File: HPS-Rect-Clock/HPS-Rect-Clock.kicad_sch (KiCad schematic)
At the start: 22 parts, among them J1 Conn_01x06, J2 PJ-102AH, Y1 Crystal_16MHz

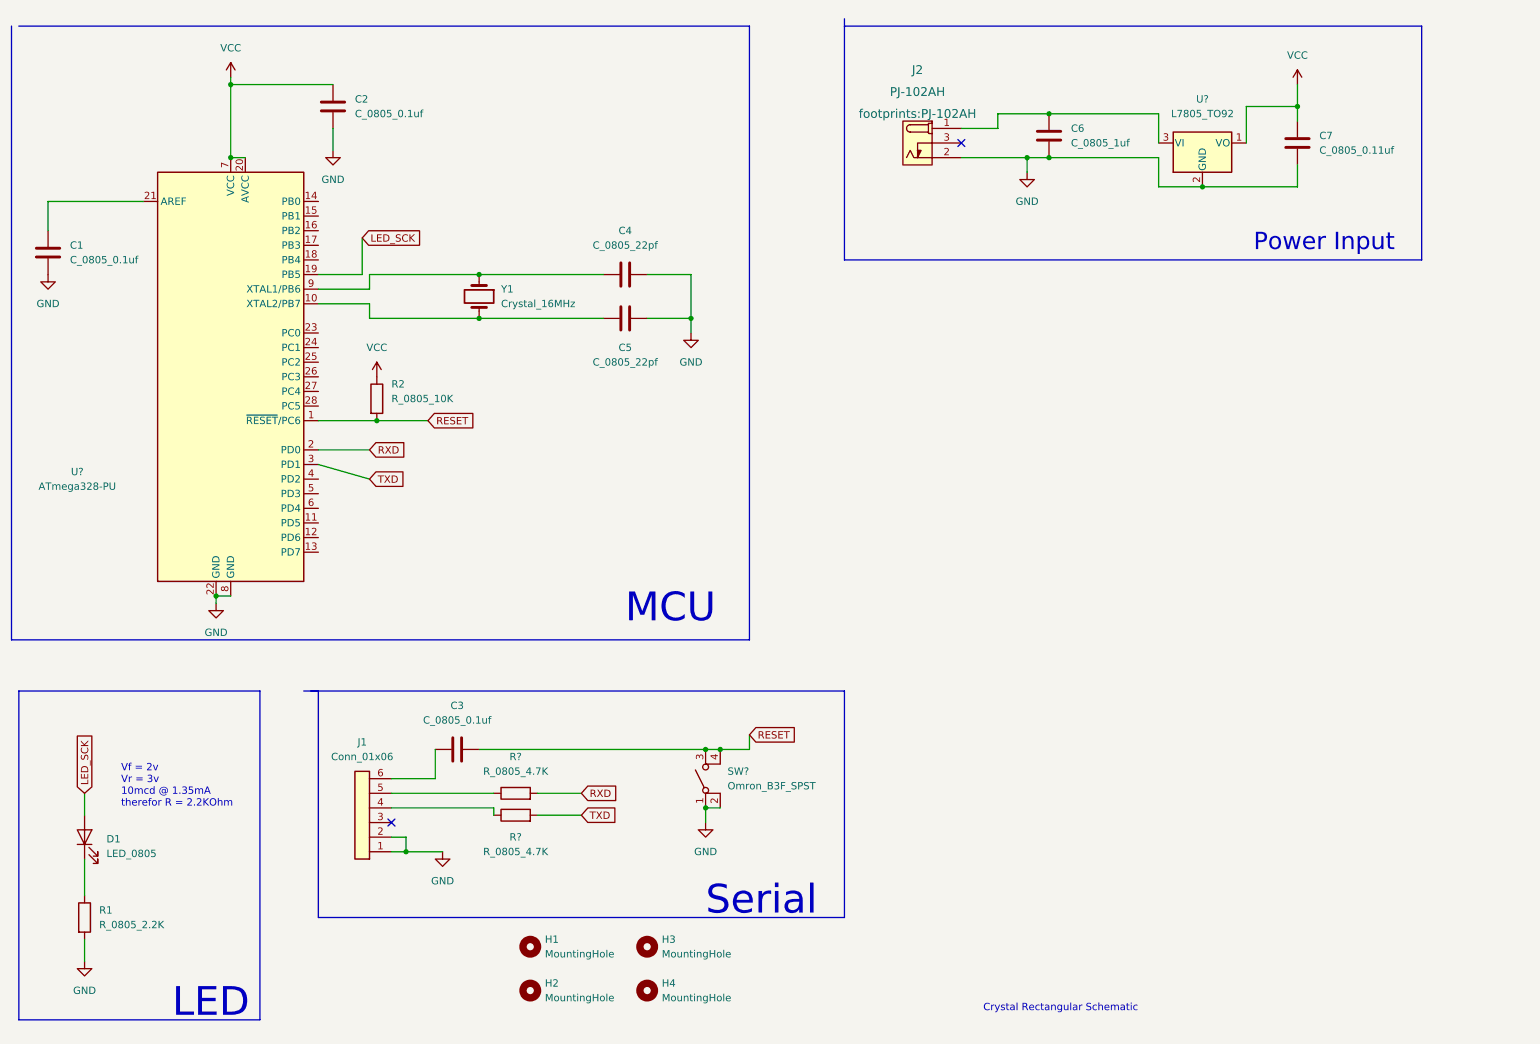
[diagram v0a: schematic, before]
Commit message: Week 3
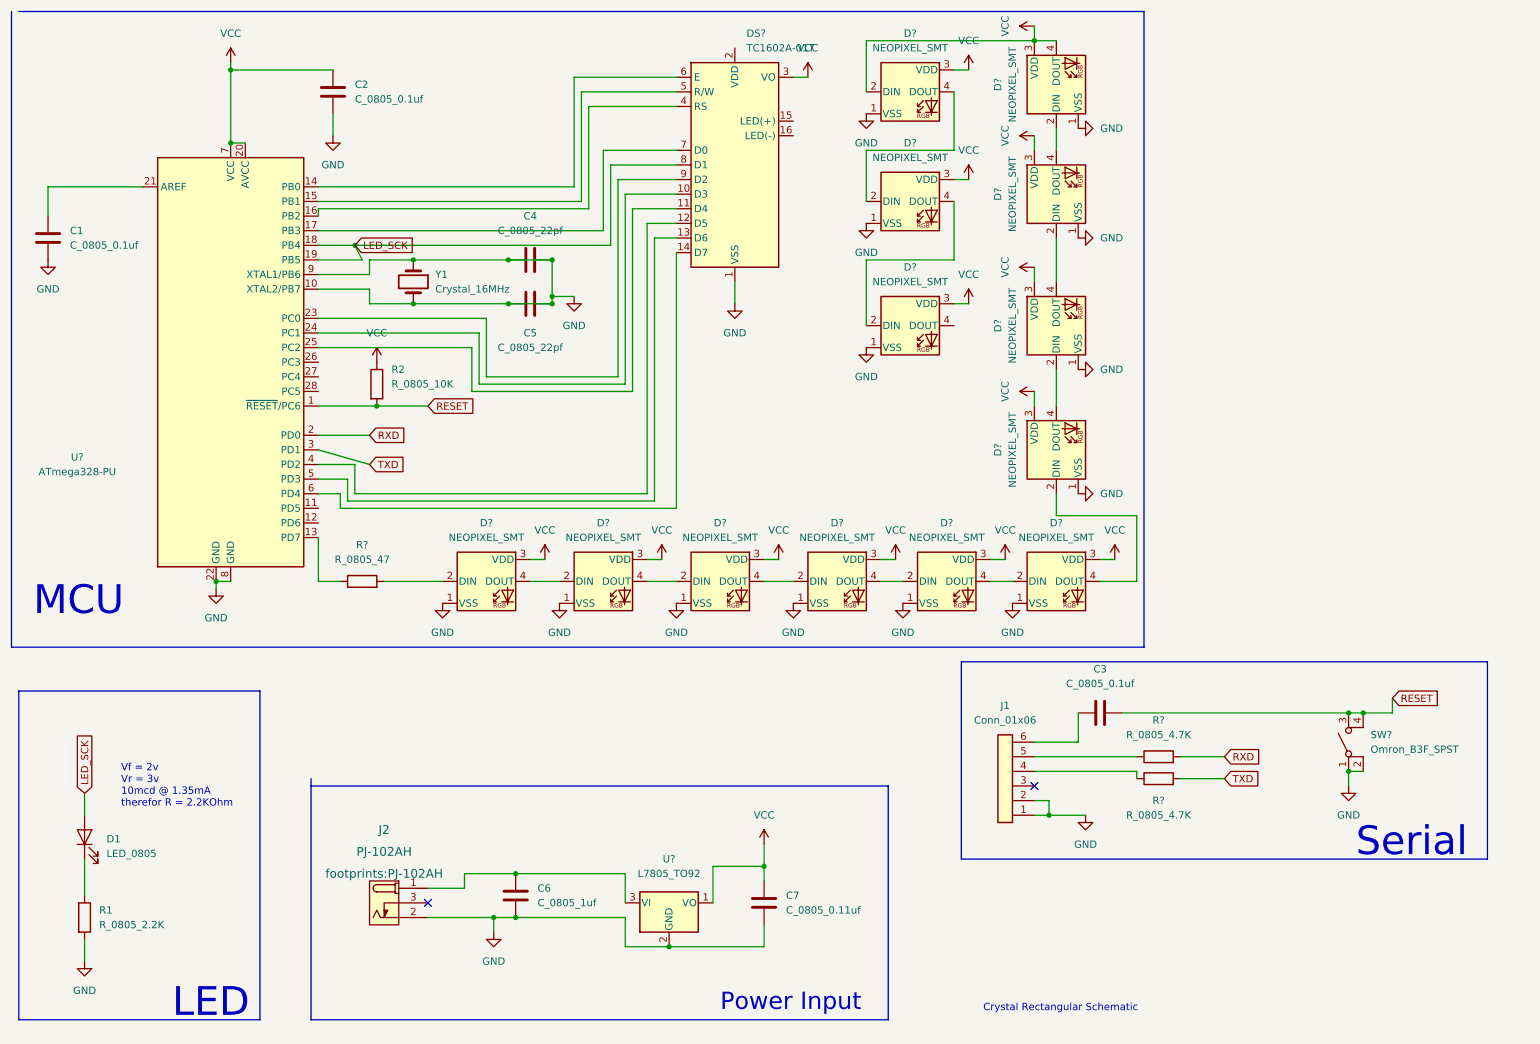
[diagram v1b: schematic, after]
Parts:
- removed H1, H2, H3, H4: MountingHole, footprints:MountingHole_3.2mm_M3, symbol HPS:MountingHole
- added D? (x13): NEOPIXEL_SMT, footprints:LED_SK6812_PLCC4_5.0x5.0mm_P3.2mm, symbol HPS:NEOPIXEL_SMT
- added DS?: TC1602A-01T, footprints:TC1602A-01T, symbol HPS:TC1602A-01T
- added R?: R_0805_47, footprints:R_0805_2012Metric, symbol HPS:R_0805_47
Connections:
- net GND: now also C4.1, C5.1, U?.10 (XTAL2/PB7), U?.9 (XTAL1/PB6), Y1.1, Y1.2, D?.1 (VSS), D?.1 (VSS), D?.1 (VSS), D?.1 (VSS), D?.1 (VSS), D?.1 (VSS), D?.1 (VSS), D?.1 (VSS), D?.1 (VSS), D?.1 (VSS), D?.1 (VSS), D?.1 (VSS), D?.1 (VSS), DS?.1 (VSS)
- net LED_SCK: now also U?.18 (PB4), DS?.8 (D1)
- net VCC: now also D?.2 (DIN), D?.3 (VDD), D?.3 (VDD), D?.3 (VDD), D?.3 (VDD), D?.3 (VDD), D?.3 (VDD), D?.3 (VDD), D?.3 (VDD), D?.3 (VDD), D?.3 (VDD), D?.3 (VDD), D?.3 (VDD), D?.3 (VDD), D?.4 (DOUT), DS?.3 (VO)
- net at U?.13 (PD7): now also R?.1
- net at U?.14 (PB0): now also DS?.6 (E)
- net at U?.15 (PB1): now also DS?.5 (R/W)
- net at U?.16 (PB2): now also DS?.4 (RS)
- net at U?.17 (PB3): now also DS?.7 (D0)
- net at U?.23 (PC0): now also DS?.9 (D2)
- net at U?.24 (PC1): now also DS?.10 (D3)
- net at U?.25 (PC2): now also DS?.11 (D4)
- net at U?.4 (PD2): now also DS?.12 (D5)
- net at U?.5 (PD3): now also DS?.13 (D6)
- net at U?.6 (PD4): now also DS?.14 (D7)
- new net: D?.2 (DIN), D?.4 (DOUT) (x11)
- new net: D?.2 (DIN), R?.2
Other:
- moved on the sheet: C1, C2, C3, C4, C5, C6, C7, J1, J2, R2, R?, SW?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
